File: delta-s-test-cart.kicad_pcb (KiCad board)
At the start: 2 copper layers, 95 x 67.5 mm, 11 parts, among them J1 SNP, J2 ZXBUS, SW1 Rom Switch, SW2 RESET, U1 74HCT32, U2 27C512

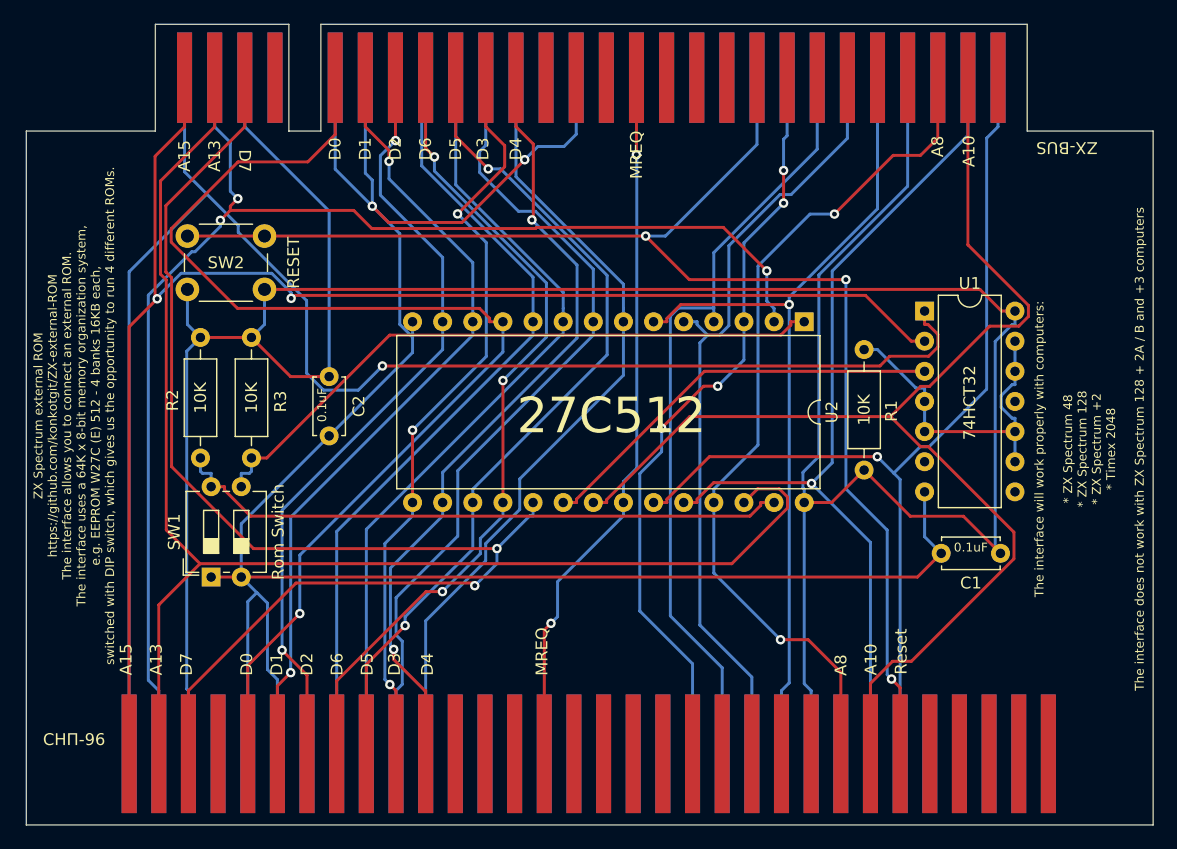
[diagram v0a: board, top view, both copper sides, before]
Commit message: Fixing stuff
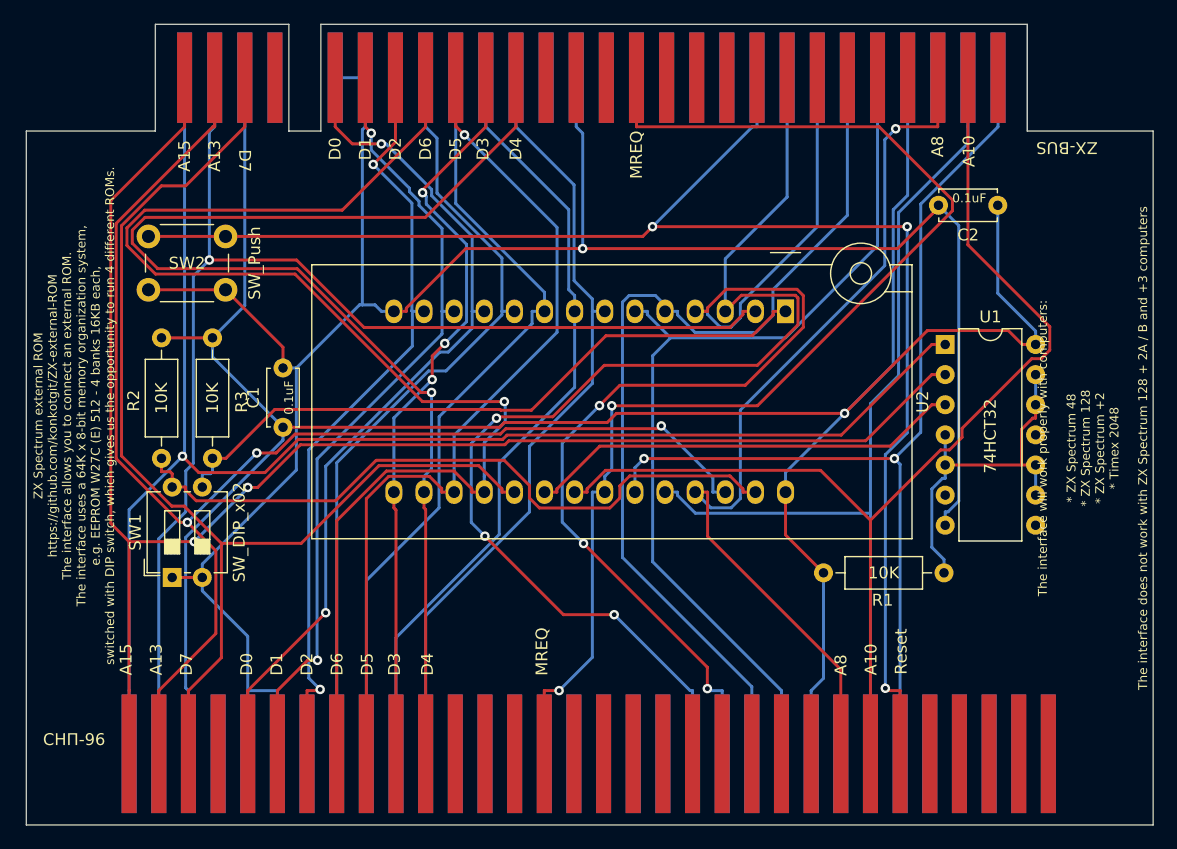
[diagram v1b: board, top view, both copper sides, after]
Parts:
- C1, C2: footprint Capacitor_THT:C_Disc_D4.7mm_W2.5mm_P5.00mm -> Diagnostic_board:C_Disc_D4.7mm_W2.5mm_P5.00mm
- J1: footprint w_conn_av:SNP96 -> Diagnostic_board:SNP96
- J2: footprint w_conn_av:ZX SPECTRUM EDGE CONNECTOR (HORIZONTAL) -> Diagnostic_board:ZX SPECTRUM EDGE CONNECTOR (HORIZONTAL)
- R1, R2, R3: footprint Resistor_THT:R_Axial_DIN0207_L6.3mm_D2.5mm_P10.16mm_Horizontal -> Diagnostic_board:R_Axial_DIN0207_L6.3mm_D2.5mm_P10.16mm_Horizontal
- SW1: value Rom Switch -> SW_DIP_x02; footprint Button_Switch_THT:SW_DIP_SPSTx02_Slide_6.7x6.64mm_W7.62mm_P2.54mm_LowProfile -> Diagnostic_board:SW_DIP_SPSTx02_Slide_6.7x6.64mm_W7.62mm_P2.54mm_LowProfile
- SW2: value RESET -> SW_Push; footprint Button_Switch_THT:SW_PUSH_6mm -> Diagnostic_board:SW_PUSH_6mm
- U1: footprint Package_DIP:DIP-14_W7.62mm -> Diagnostic_board:DIP-14_W7.62mm
- U2: footprint Package_DIP:DIP-28_W15.24mm -> Socket:DIP_Socket-28_W11.9_W12.7_W15.24_W17.78_W18.5_3M_228-1277-00-0602J
- moved C1 61.4 mm to (105.3, 79.5), turned to 90 degrees
- moved C2 58.2 mm to (165.6, 60.8), turned to 180 degrees
- moved R1 9.32 mm to (150.9, 91.7), turned to 0 degrees
- moved U1 3.31 mm to (161.1, 72.5)
- moved R3 3.29 mm to (99.4, 71.9)
- moved SW1 3.29 mm to (96.0, 92.1)
- moved SW2 3.29 mm to (94.0, 63.4)
- moved R2 3.29 mm to (95.1, 71.9)
- moved U2 1.80 mm to (147.7, 69.7)
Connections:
- SW2 pad 2: +5V -> GND
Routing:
- net D6: track 69.4 -> 114.7 mm, vias 3 -> 1
- net MREQ: track 60.2 -> 102.8 mm
- net +5V: track 252.0 -> 211.8 mm, vias 0 -> 1
- net D4: track 67.0 -> 102.4 mm, vias 2 -> 1
- net A7: track 64.7 -> 99.1 mm, vias 4 -> 3
- net A6: track 66.8 -> 97.5 mm, vias 0 -> 3
- net D0: track 99.3 -> 72.7 mm, vias 1 -> 2
- net A5: track 67.7 -> 80.7 mm
- net D7: track 108.6 -> 96.3 mm, vias 2 -> 0
- net A10: track 104.6 -> 94.6 mm
- net RESET: track 117.1 -> 127.1 mm
- net A14: track 138.1 -> 128.3 mm
- net A15: track 127.6 -> 134.9 mm
- net Net-(U2-A14): track 52.5 -> 59.2 mm
- net A4: track 72.6 -> 79.1 mm, vias 1 -> 0
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
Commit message: Update
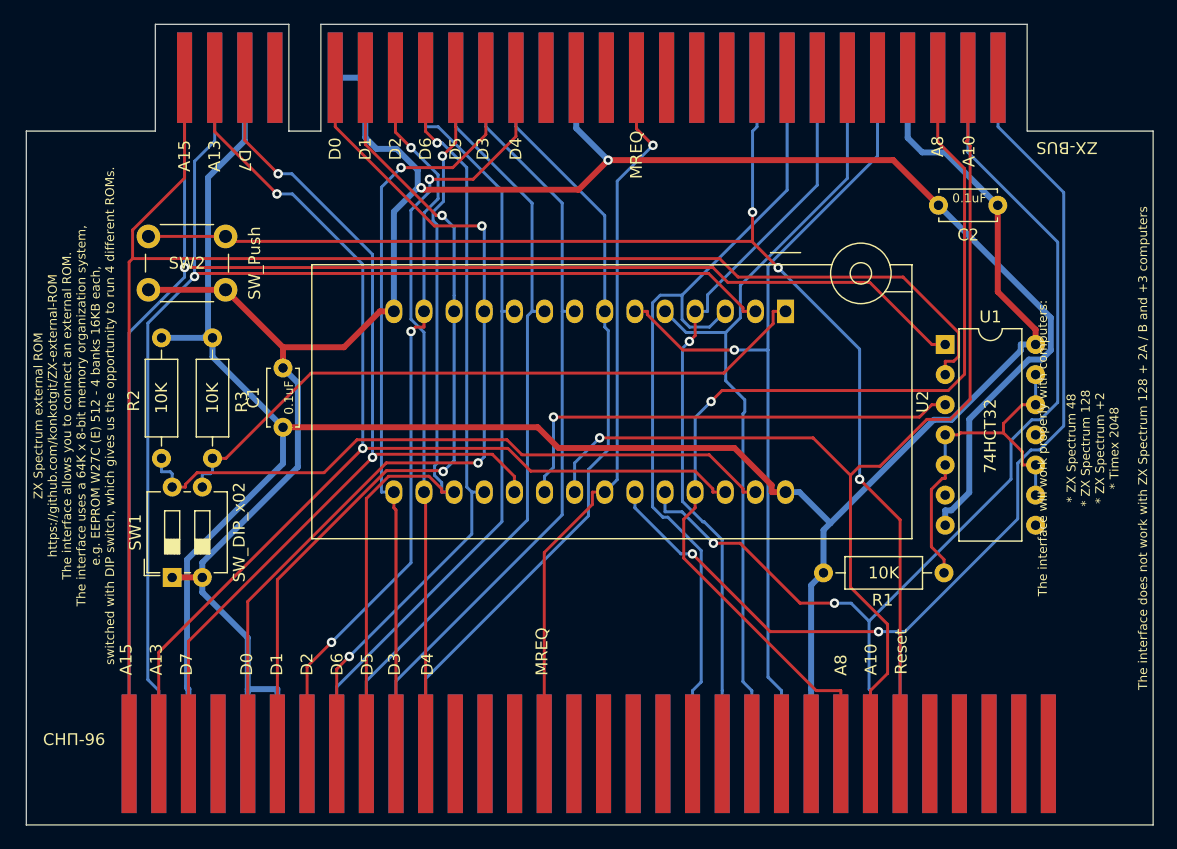
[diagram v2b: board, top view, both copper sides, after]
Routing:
- net D6: track 114.7 -> 64.6 mm, vias 1 -> 2
- net MREQ: track 102.8 -> 62.0 mm, vias 2 -> 1
- net D4: track 102.4 -> 63.4 mm
- net A6: track 97.5 -> 63.8 mm, vias 3 -> 1
- net A7: track 99.1 -> 71.5 mm, vias 3 -> 0
- net +5V: track 211.8 -> 190.3 mm, vias 1 -> 0
- net A13: track 118.1 -> 102.3 mm, vias 3 -> 2
- net RESET: track 127.1 -> 113.4 mm
- net D7: track 96.3 -> 82.7 mm, vias 0 -> 2
- net A5: track 80.7 -> 68.1 mm
- net A9: track 78.6 -> 89.9 mm, vias 0 -> 2
- net A8: track 76.8 -> 85.6 mm
- net A11: track 85.1 -> 93.7 mm
- net A4: track 79.1 -> 74.0 mm, vias 0 -> 1
- net D5: track 72.5 -> 67.7 mm
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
